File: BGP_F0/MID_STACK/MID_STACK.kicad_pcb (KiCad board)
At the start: 2 copper layers, 20 x 26 mm, 7 parts, among them P1 CONN_01X04, P2 CONN_01X09

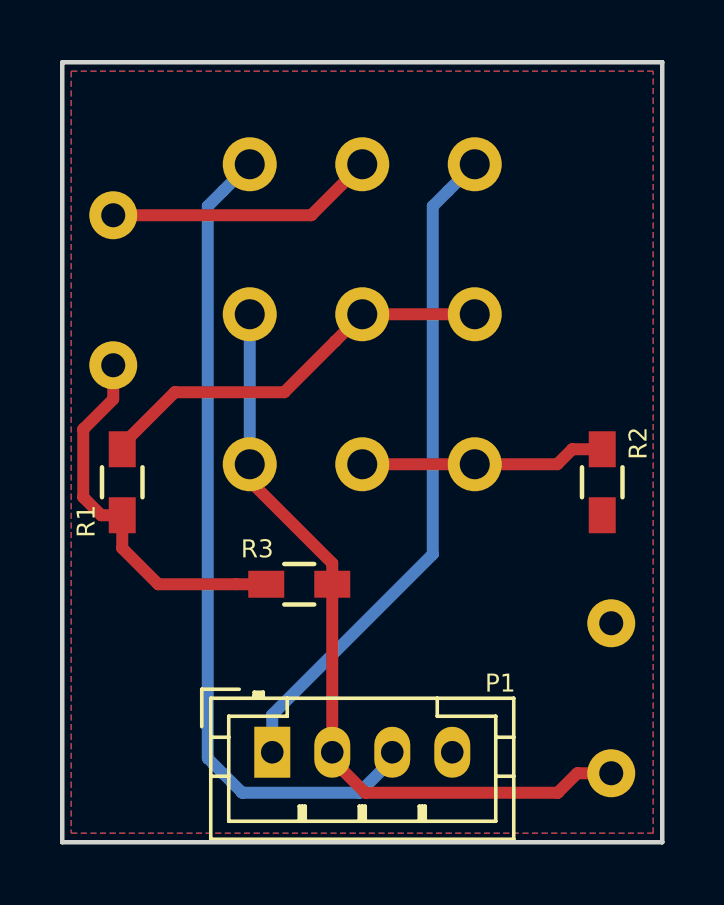
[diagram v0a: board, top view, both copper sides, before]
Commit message: Mods and gerbers done
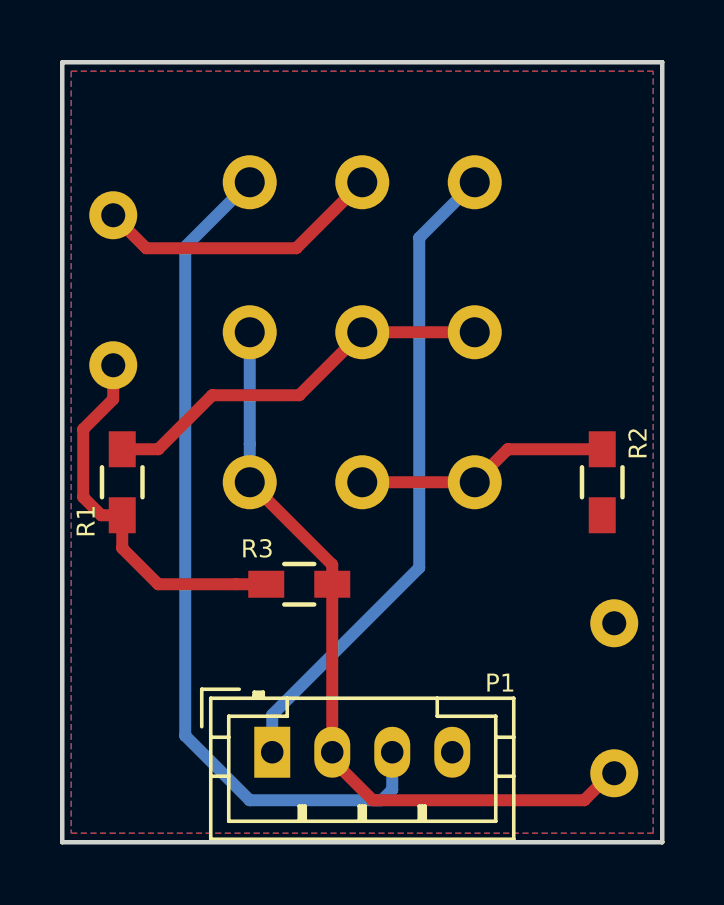
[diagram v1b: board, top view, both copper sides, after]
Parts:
- moved P2 0.60 mm to (171.2, 96.0)
- moved C2 0.10 mm to (183.4, 115.7)
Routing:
- net /MID_O: track 27.7 -> 28.8 mm
- net /VOL2: track 9.00 -> 9.67 mm
- net /MID_I: track 22.6 -> 22.0 mm
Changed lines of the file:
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@@
     (thickness 1.6)
     (drawings 8)
-    (tracks 46)
+    (tracks 44)
     (zones 0)
     (modules 7)
@@
     (visible_elements 7FFFFFFF)
     (pcbplotparams
-      (layerselection 0x010f0_80000001)
+      (layerselection 0x010fc_80000001)
       (usegerberextensions true)
       (usegerberattributes true)
@@
       (drillshape 0)
       (scaleselection 1)
-      (outputdirectory ../../GERBER/MID_0/))
+      (outputdirectory ../../GERBER/F0_MID/))
   )
   (net 0 "")
@@
   )
   (module LIBS:Potentiometer_Alpha_Tripple_Vertical_Dual_Shaft (layer B.Cu)
-    (at 171.25 95.4 90)
+    (at 171.25 96 90)
     (descr "Potentiometer, vertically mounted, Omeg PC16PU, Omeg PC16PU, Omeg PC16PU, Vishay/Spectrol 248GJ/249GJ Single, Vishay/Spectrol 248GJ/249GJ Single, Vishay/Spectrol 248GJ/249GJ Single, Vishay/Spectrol 248GH/249GH Single, Vishay/Spectrol 148/149 Single, Vishay/Spectrol 148/149 Single, Vishay/Spectrol 148/149 Single, Vishay/Spectrol 148A/149A Single with mounting plates, Vishay/Spectrol 148/149 Double, Vishay/Spectrol 148A/149A Double with mounting plates, Piher PC-16 Single, Piher PC-16 Single, Piher PC-16 Single, Piher PC-16SV Single, Piher PC-16 Double, Piher PC-16 Triple, Piher T16H Single, Piher T16L Single, Piher T16H Double, Alps RK163 Single, Alps RK163 Double, Alps RK097 Single, Alps RK097 Double, http://www.alps.com/prod/info/E/HTML/Potentiometer/RotaryPotentiometers/RK097/RK09712100AV.html")
     (tags "Potentiometer vertical  Omeg PC16PU  Omeg PC16PU  Omeg PC16PU  Vishay/Spectrol 248GJ/249GJ Single  Vishay/Spectrol 248GJ/249GJ Single  Vishay/Spectrol 248GJ/249GJ Single  Vishay/Spectrol 248GH/249GH Single  Vishay/Spectrol 148/149 Single  Vishay/Spectrol 148/149 Single  Vishay/Spectrol 148/149 Single  Vishay/Spectrol 148A/149A Single with mounting plates  Vishay/Spectrol 148/149 Double  Vishay/Spectrol 148A/149A Double with mounting plates  Piher PC-16 Single  Piher PC-16 Single  Piher PC-16 Single  Piher PC-16SV Single  Piher PC-16 Double  Piher PC-16 Triple  Piher T16H Single  Piher T16L Single  Piher T16H Double  Alps RK163 Single  Alps RK163 Double  Alps RK097 Single  Alps RK097 Double Dual Shaft")
@@
   )
   (module Capacitor_THT:C_Rect_L7.2mm_W2.5mm_P5.00mm_FKS2_FKP2_MKS2_MKP2 (layer B.Cu)
-    (at 183.3 115.7 90)
+    (at 183.4 115.7 90)
     (descr "C, Rect series, Radial, pin pitch=5.00mm, length*width=7.2*2.5mm^2, Capacitor, http://www.wima.com/EN/WIMA_FKS_2.pdf")
     (tags "C Rect series Radial pin pitch 5.00mm  length 7.2mm width 2.5mm Capacitor")
@@
   (gr_line (start 165 92) (end 165 118) (layer Edge.Cuts) (width 0.15))
   (gr_line (start 185 92) (end 165 92) (layer Edge.Cuts) (width 0.15))
-  (segment (start 166.7 97.1) (end 173.3 97.1) (width 0.4) (layer F.Cu) (net 1))
-  (segment (start 173.3 97.1) (end 175 95.4) (width 0.4) (layer F.Cu) (net 1))
+  (segment (start 172.8 98.2) (end 167.8 98.2) (width 0.4) (layer F.Cu) (net 1))
+  (segment (start 167.8 98.2) (end 166.7 97.1) (width 0.4) (layer F.Cu) (net 1))
+  (segment (start 175 96) (end 172.8 98.2) (width 0.4) (layer F.Cu) (net 1))
   (segment (start 166.7 102.1) (end 166.7 103.23137) (width 0.4) (layer F.Cu) (net 2))
   (segment (start 166.7 103.23137) (end 165.7 104.23137) (width 0.4) (layer F.Cu) (net 2))
@@
   (segment (start 168.2 109.4) (end 170.8 109.4) (width 0.4) (layer F.Cu) (net 2))
   (segment (start 170.8 109.4) (end 171.8 109.4) (width 0.4) (layer F.Cu) (net 2))
-  (segment (start 171.25 106) (end 171.25 101) (width 0.4) (layer B.Cu) (net 3))
-  (segment (start 171.3 101.05) (end 171.35 101) (width 0.4) (layer B.Cu) (net 3))
-  (segment (start 174 109.4) (end 174 108.7) (width 0.4) (layer F.Cu) (net 3))
-  (segment (start 174 108.7) (end 171.3 106) (width 0.4) (layer F.Cu) (net 3))
+  (segment (start 183.3 115.7) (end 182.4 116.6) (width 0.4) (layer F.Cu) (net 3))
+  (segment (start 182.4 116.6) (end 175.35 116.6) (width 0.4) (layer F.Cu) (net 3))
+  (segment (start 175.35 116.6) (end 174 115.25) (width 0.4) (layer F.Cu) (net 3))
+  (segment (start 174 115.25) (end 174 115) (width 0.4) (layer F.Cu) (net 3))
+  (segment (start 171.25 106) (end 171.25 104.727208) (width 0.4) (layer B.Cu) (net 3))
+  (segment (start 171.25 104.727208) (end 171.25 101) (width 0.4) (layer B.Cu) (net 3))
+  (segment (start 171.25 106) (end 174 108.75) (width 0.4) (layer F.Cu) (net 3))
+  (segment (start 174 108.75) (end 174 109.4) (width 0.4) (layer F.Cu) (net 3))
   (segment (start 171.3 106) (end 171.25 106) (width 0.4) (layer F.Cu) (net 3))
-  (segment (start 183.3 115.7) (end 182.16863 115.7) (width 0.4) (layer F.Cu) (net 3))
-  (segment (start 182.16863 115.7) (end 181.51862 116.35001) (width 0.4) (layer F.Cu) (net 3))
-  (segment (start 181.51862 116.35001) (end 175.10001 116.35001) (width 0.4) (layer F.Cu) (net 3))
-  (segment (start 175.10001 116.35001) (end 174 115.25) (width 0.4) (layer F.Cu) (net 3))
-  (segment (start 174 115.25) (end 174 115) (width 0.4) (layer F.Cu) (net 3))
   (segment (start 174 115) (end 174 109.4) (width 0.4) (layer F.Cu) (net 3))
   (segment (start 178 114.75) (end 178 115) (width 0.4) (layer B.Cu) (net 4))
+  (segment (start 176.9 108.85) (end 176.9 97.85) (width 0.4) (layer B.Cu) (net 5))
+  (segment (start 176.9 97.85) (end 178.75 96) (width 0.4) (layer B.Cu) (net 5))
   (segment (start 172 115) (end 172 113.75) (width 0.4) (layer B.Cu) (net 5))
-  (segment (start 172 113.75) (end 177.349999 108.400001) (width 0.4) (layer B.Cu) (net 5))
-  (segment (start 177.349999 96.800001) (end 177.850001 96.299999) (width 0.4) (layer B.Cu) (net 5))
-  (segment (start 177.349999 108.400001) (end 177.349999 96.800001) (width 0.4) (layer B.Cu) (net 5))
-  (segment (start 177.850001 96.299999) (end 178.75 95.4) (width 0.4) (layer B.Cu) (net 5))
+  (segment (start 172 113.75) (end 176.9 108.85) (width 0.4) (layer B.Cu) (net 5))
   (segment (start 172 115) (end 172 114.75) (width 0.4) (layer B.Cu) (net 5))
+  (segment (start 176 115) (end 176 116.25) (width 0.4) (layer B.Cu) (net 6))
+  (segment (start 176 116.25) (end 175.65 116.6) (width 0.4) (layer B.Cu) (net 6))
+  (segment (start 175.65 116.6) (end 171.249998 116.6) (width 0.4) (layer B.Cu) (net 6))
+  (segment (start 171.249998 116.6) (end 169.1 114.450002) (width 0.4) (layer B.Cu) (net 6))
+  (segment (start 169.1 114.450002) (end 169.1 98.15) (width 0.4) (layer B.Cu) (net 6))
+  (segment (start 169.1 98.15) (end 171.25 96) (width 0.4) (layer B.Cu) (net 6))
   (segment (start 176 115) (end 176 115.25) (width 0.4) (layer B.Cu) (net 6))
-  (segment (start 176 115.25) (end 174.899999 116.350001) (width 0.4) (layer B.Cu) (net 6))
-  (segment (start 170.350001 96.299999) (end 171.25 95.4) (width 0.4) (layer B.Cu) (net 6))
-  (segment (start 174.899999 116.350001) (end 170.999999 116.350001) (width 0.4) (layer B.Cu) (net 6))
-  (segment (start 170.999999 116.350001) (end 169.849999 115.200001) (width 0.4) (layer B.Cu) (net 6))
-  (segment (start 169.849999 115.200001) (end 169.849999 96.800001) (width 0.4) (layer B.Cu) (net 6))
-  (segment (start 169.849999 96.800001) (end 170.350001 96.299999) (width 0.4) (layer B.Cu) (net 6))
+  (segment (start 175 101) (end 178.75 101) (width 0.4) (layer F.Cu) (net 7))
+  (segment (start 170 103.1) (end 172.9 103.1) (width 0.4) (layer F.Cu) (net 7))
+  (segment (start 172.9 103.1) (end 175 101) (width 0.4) (layer F.Cu) (net 7))
+  (segment (start 168.2 104.9) (end 170 103.1) (width 0.4) (layer F.Cu) (net 7))
+  (segment (start 167 104.9) (end 168.2 104.9) (width 0.4) (layer F.Cu) (net 7))
   (segment (start 167 104.9) (end 167 104.75) (width 0.4) (layer F.Cu) (net 7))
-  (segment (start 167 104.75) (end 168.75 103) (width 0.4) (layer F.Cu) (net 7))
-  (segment (start 168.75 103) (end 172.4 103) (width 0.4) (layer F.Cu) (net 7))
-  (segment (start 174.100001 101.299999) (end 175 100.4) (width 0.4) (layer F.Cu) (net 7))
-  (segment (start 172.4 103) (end 174.100001 101.299999) (width 0.4) (layer F.Cu) (net 7))
-  (segment (start 178.75 100.4) (end 175 100.4) (width 0.4) (layer F.Cu) (net 7))
-  (segment (start 178.75 105.4) (end 175 105.4) (width 0.4) (layer F.Cu) (net 8))
-  (segment (start 183 104.9) (end 182 104.9) (width 0.4) (layer F.Cu) (net 8))
-  (segment (start 182 104.9) (end 181.5 105.4) (width 0.4) (layer F.Cu) (net 8))
-  (segment (start 181.5 105.4) (end 178.75 105.4) (width 0.4) (layer F.Cu) (net 8))
+  (segment (start 183 104.9) (end 179.85 104.9) (width 0.4) (layer F.Cu) (net 8))
+  (segment (start 179.85 104.9) (end 178.75 106) (width 0.4) (layer F.Cu) (net 8))
+  (segment (start 175 106) (end 178.75 106) (width 0.4) (layer F.Cu) (net 8))
   (zone (net 4) (net_name /Vref) (layer F.Cu) (hatch edge 0.508)
     (connect_pads (clearance 0.3))
